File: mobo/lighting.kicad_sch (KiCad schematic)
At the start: 4 parts, among them J106 Conn_01x03, J108 Conn_01x03, U18 SN74LVC2G34, U22 PESD5V2S2UT

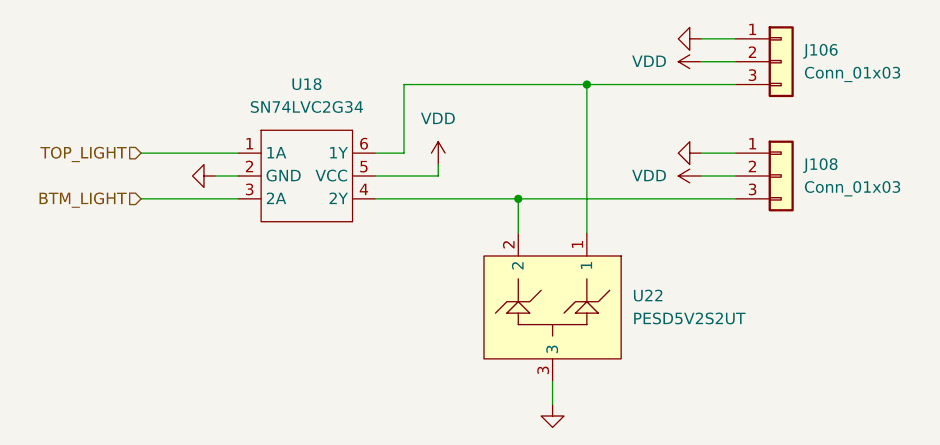
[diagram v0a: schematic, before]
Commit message: mobo v1, 1 unit
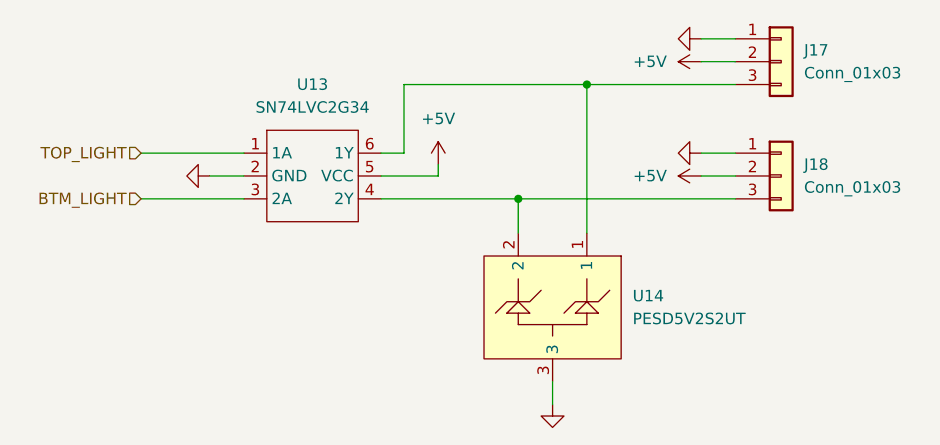
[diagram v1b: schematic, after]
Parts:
- J17: renamed from J106; footprint (none) -> mobo:JST_PH_B3B-PH-SM4-TB_1x03-1MP_P2.00mm_Vertical
- J18: renamed from J108; footprint (none) -> mobo:JST_PH_B3B-PH-SM4-TB_1x03-1MP_P2.00mm_Vertical
- renumbered U18 to U13, U22 to U14
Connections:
- net VDD renamed +5V
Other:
- moved on the sheet: U13
